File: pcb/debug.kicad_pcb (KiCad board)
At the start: 2 copper layers, 65 parts, among them J1 Val**, J2 USB_C_Receptacle_USB2.0, Q1 Q_PNP_BCE, SW1 SW_DIP_x02, SW2 Reset, U1 STLQ020PU33R, U2 FT4222HQ, U3 STM32F103V8Tx, U4 INA381AxDSG, U5 SN74ALVC00, U6 MIC94090, Y1 12MHz, Y2 24MHz

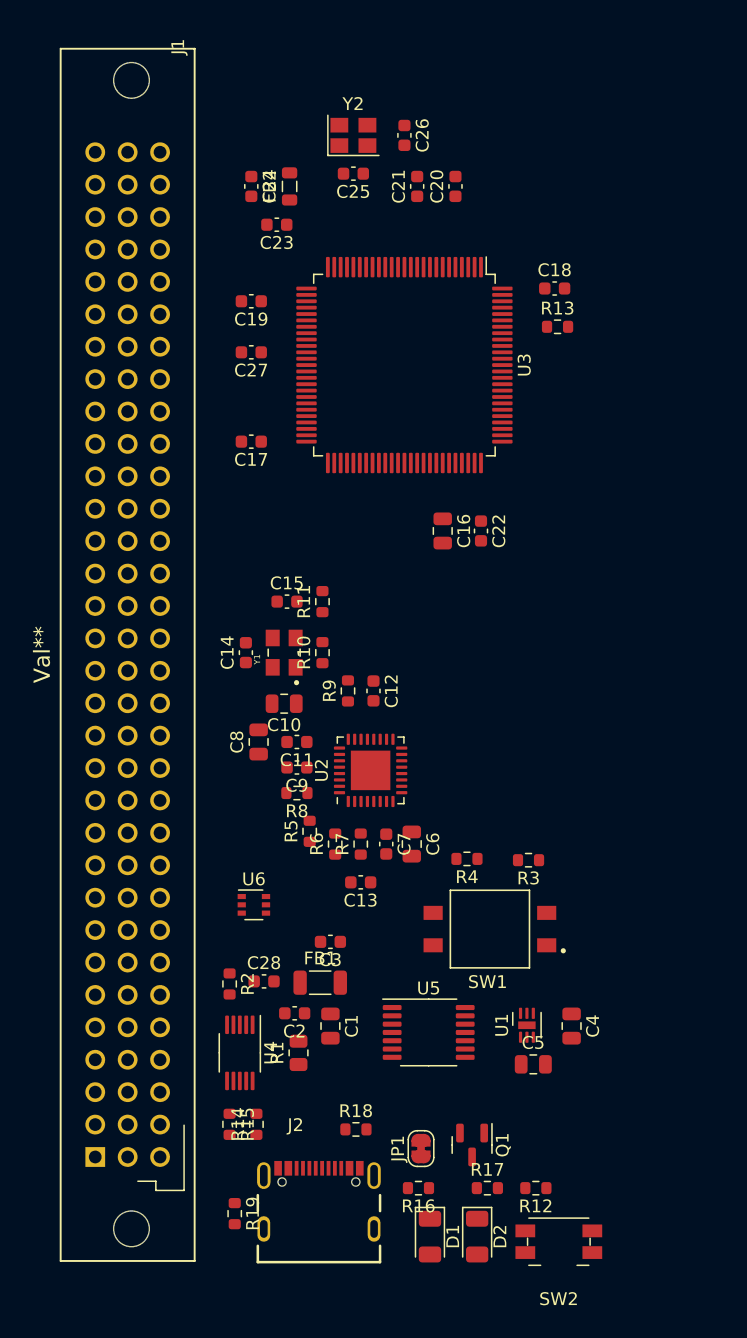
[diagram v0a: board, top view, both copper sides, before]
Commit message: finished placing components
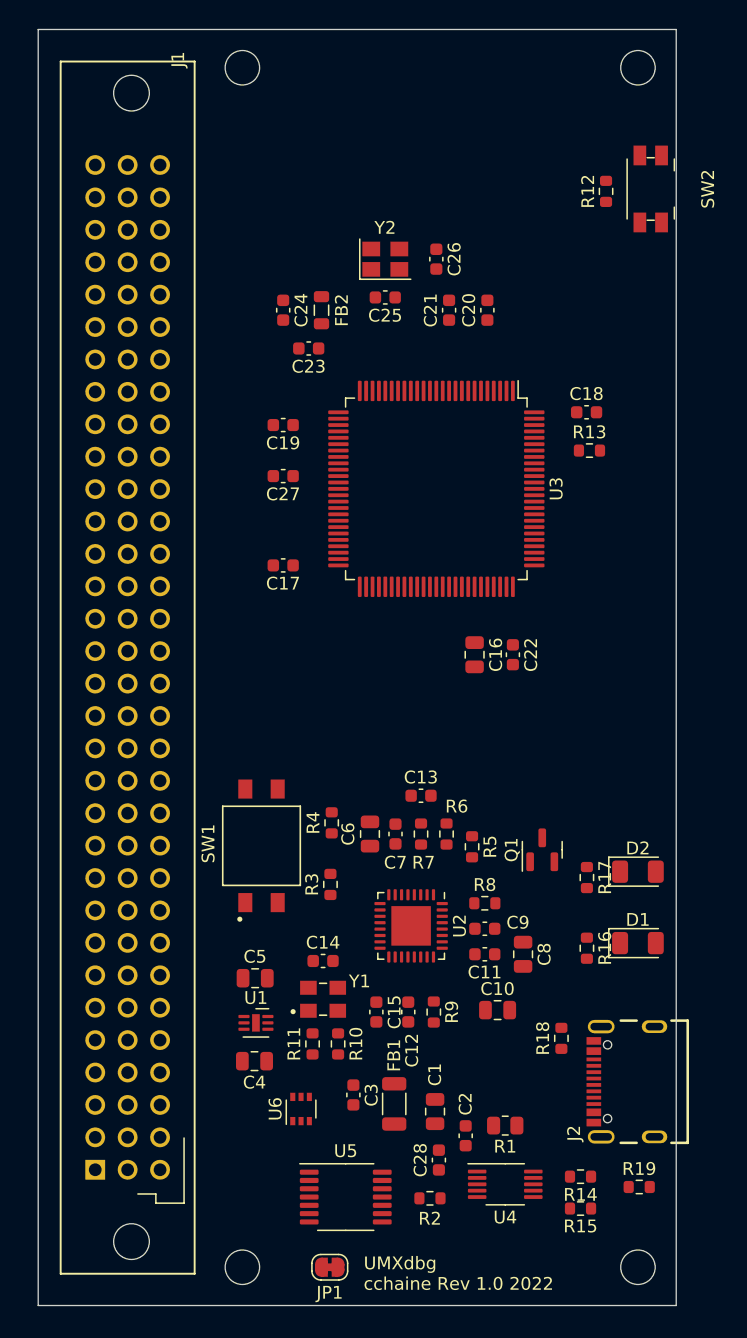
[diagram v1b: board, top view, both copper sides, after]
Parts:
- added H1: MountingHole, MountingHole:MountingHole_2.7mm_M2.5, F.Cu at (95.0, 52.0)
- added H2: MountingHole, MountingHole:MountingHole_2.7mm_M2.5, F.Cu at (95.0, 146.0)
- added H3: MountingHole, MountingHole:MountingHole_2.7mm_M2.5, F.Cu at (126.0, 146.0)
- added H4: MountingHole, MountingHole:MountingHole_2.7mm_M2.5, F.Cu at (126.0, 52.0)
- J1: value Val** -> 09032967825
- moved SW2 82.8 mm to (127.0, 61.5), turned to -90 degrees
- moved R12 78.3 mm to (123.5, 61.7), turned to -90 degrees
- moved R11 34.7 mm to (100.5, 128.5)
- moved C15 32.9 mm to (105.5, 126.0), turned to -90 degrees
- moved R19 31.8 mm to (126.1, 139.7), turned to 0 degrees
- moved D2 31.3 mm to (126.0, 115.0), turned to 0 degrees
- moved R10 30.7 mm to (102.5, 128.5), turned to -90 degrees
- moved C10 29.3 mm to (115.0, 125.8), turned to 0 degrees
- moved J2 28.7 mm to (127.3, 131.5), turned to 90 degrees
- moved R15 28.3 mm to (121.5, 141.4), turned to 0 degrees
- moved D1 28.2 mm to (126.0, 120.6), turned to 0 degrees
- moved Y1 27.3 mm to (101.3, 125.0), turned to 0 degrees
- moved C8 26.6 mm to (117.0, 121.5), turned to -90 degrees
- moved R9 26.0 mm to (110.0, 126.0), turned to -90 degrees
- moved R14 25.7 mm to (121.5, 138.9), turned to 180 degrees
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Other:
- board outline added: 50 x 100 mm
- copper layers 2 -> 4
- board text added: "UMXdbg cchaine Rev 1.0 2022"
